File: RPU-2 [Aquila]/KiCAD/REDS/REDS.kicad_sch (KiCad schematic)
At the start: 15 parts, among them J1 Pigtail, J2 Our Power, M1 Motor_Servo, U1 MAX4543, U2 AmazonBuck, U3 LM555xN

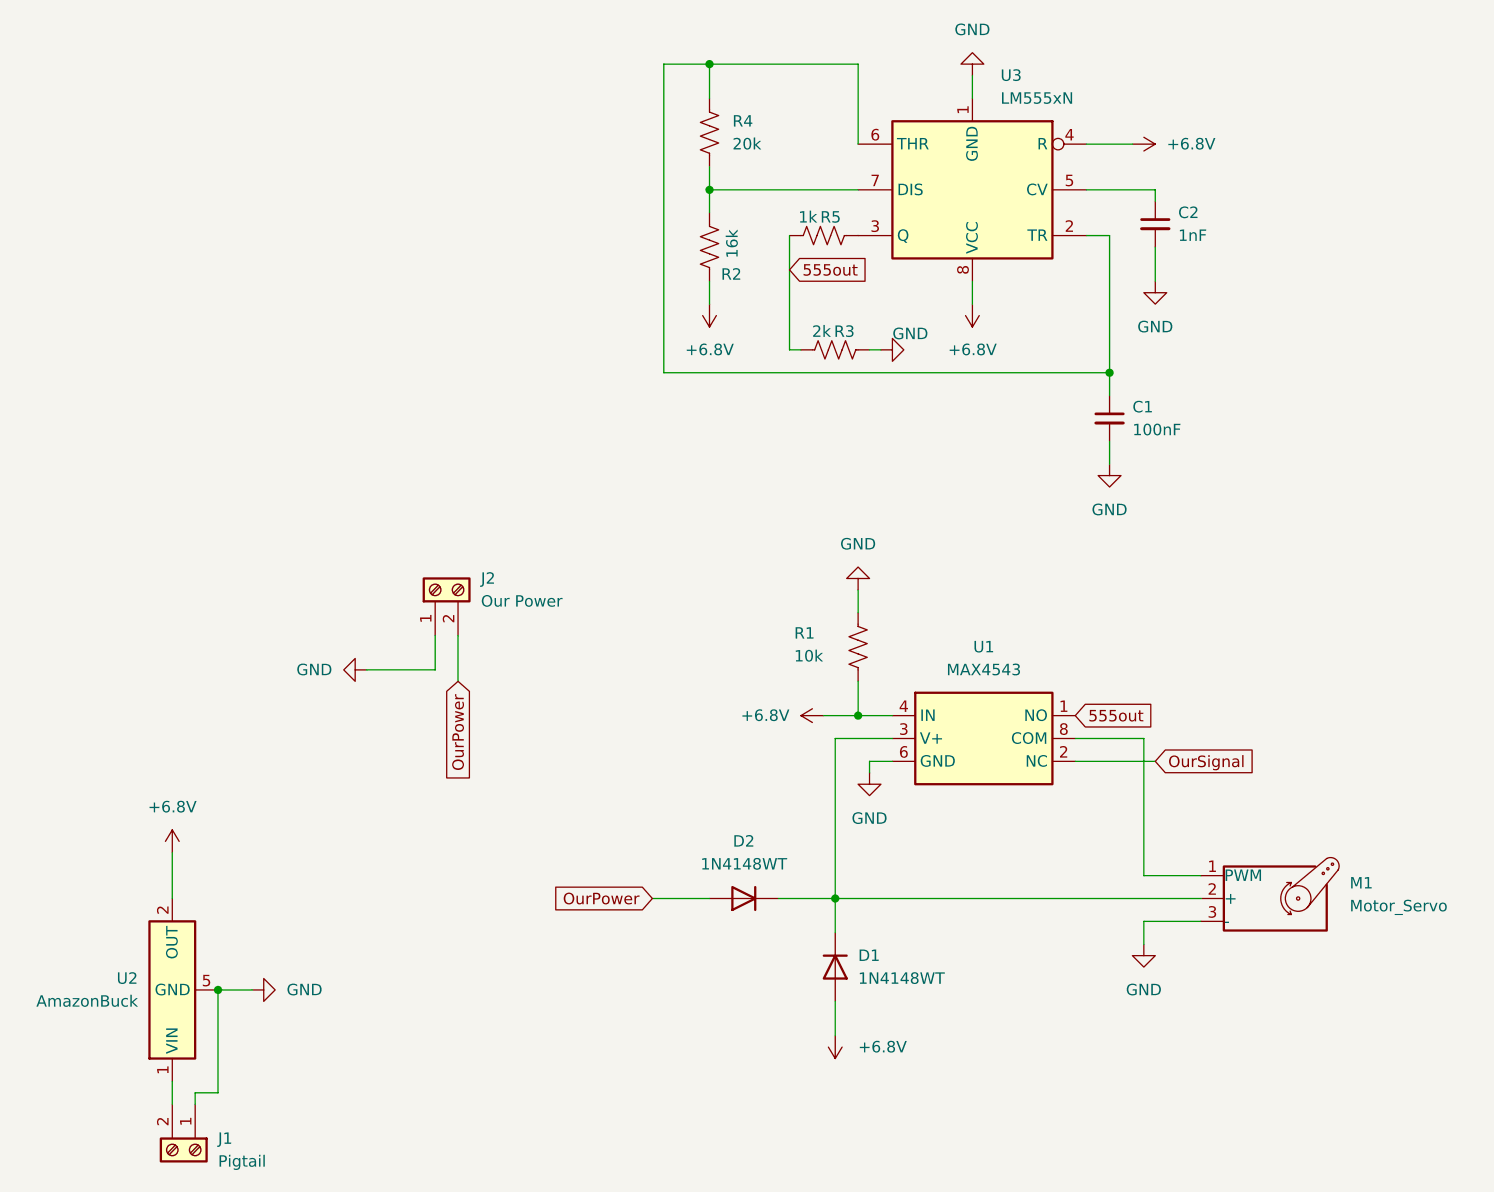
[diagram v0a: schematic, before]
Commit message: kicad updat
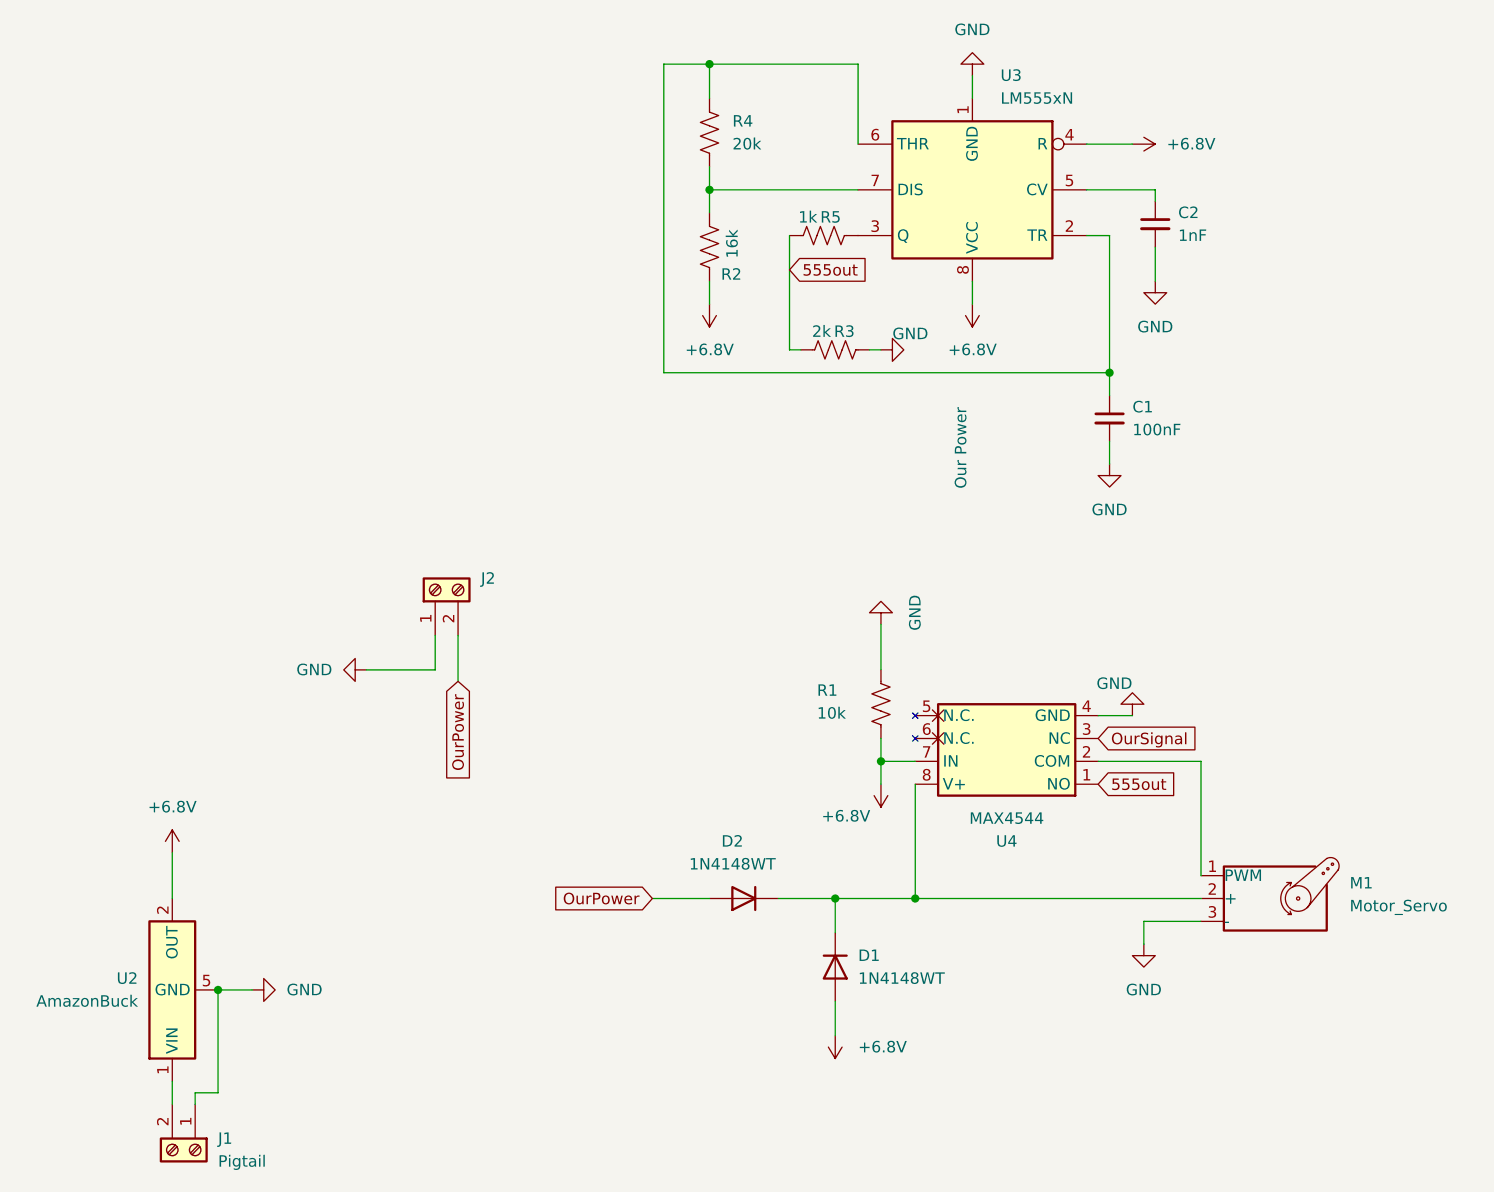
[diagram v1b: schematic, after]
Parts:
- removed U1: MAX4543, Package_DIP:DIP-8_W7.62mm, symbol MAX4543:MAX4543
- added U4: MAX4544, Package_SO:MSOP-8_3x3mm_P0.65mm, symbol MAX4543:MAX4543
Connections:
- net +6.8V: now also U4.7 (IN)
- net 555out: now also U4.1 (NO)
- net GND: now also U4.4 (GND)
- net OurSignal: now also U4.3 (NC)
- net at D1.1 (K), D2.1 (K), M1.2 (+): now also U4.8 (V+)
- net at M1.1 (PWM): now also U4.2 (COM)
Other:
- moved on the sheet: R1
